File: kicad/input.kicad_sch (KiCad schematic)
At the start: 4 parts, among them SW701 BT1, SW702 BT2, SW703 BT3, SW704 BT4

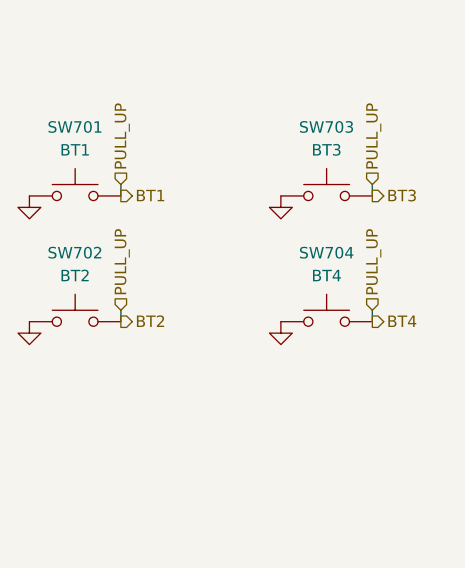
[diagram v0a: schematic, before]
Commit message: refactor, fix issues, ready for first design
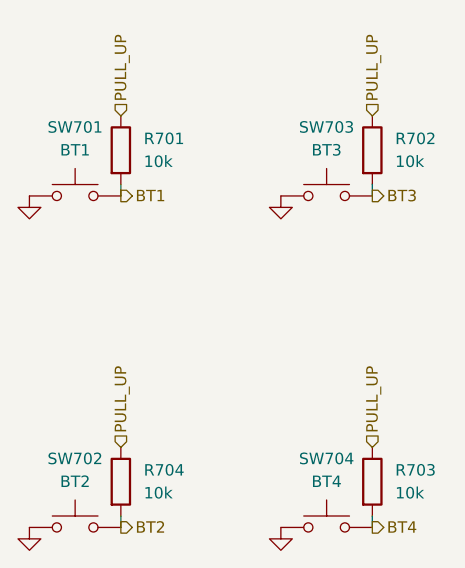
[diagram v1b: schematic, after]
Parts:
- added R701, R702, R703, R704: 10k, symbol Device:R
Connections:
- net BT1: now also R701.2; no longer SW702.2, SW703.2, SW704.2
- new net BT2: R704.2, SW702.2
- new net BT3: R702.2, SW703.2
- new net BT4: R703.2, SW704.2
- new net PULL_UP: R701.1, R702.1, R703.1, R704.1
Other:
- moved on the sheet: SW702, SW704
